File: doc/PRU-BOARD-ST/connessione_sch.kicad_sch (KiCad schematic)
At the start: 1 part, among them J1 Conn_02x25_Top_Bottom

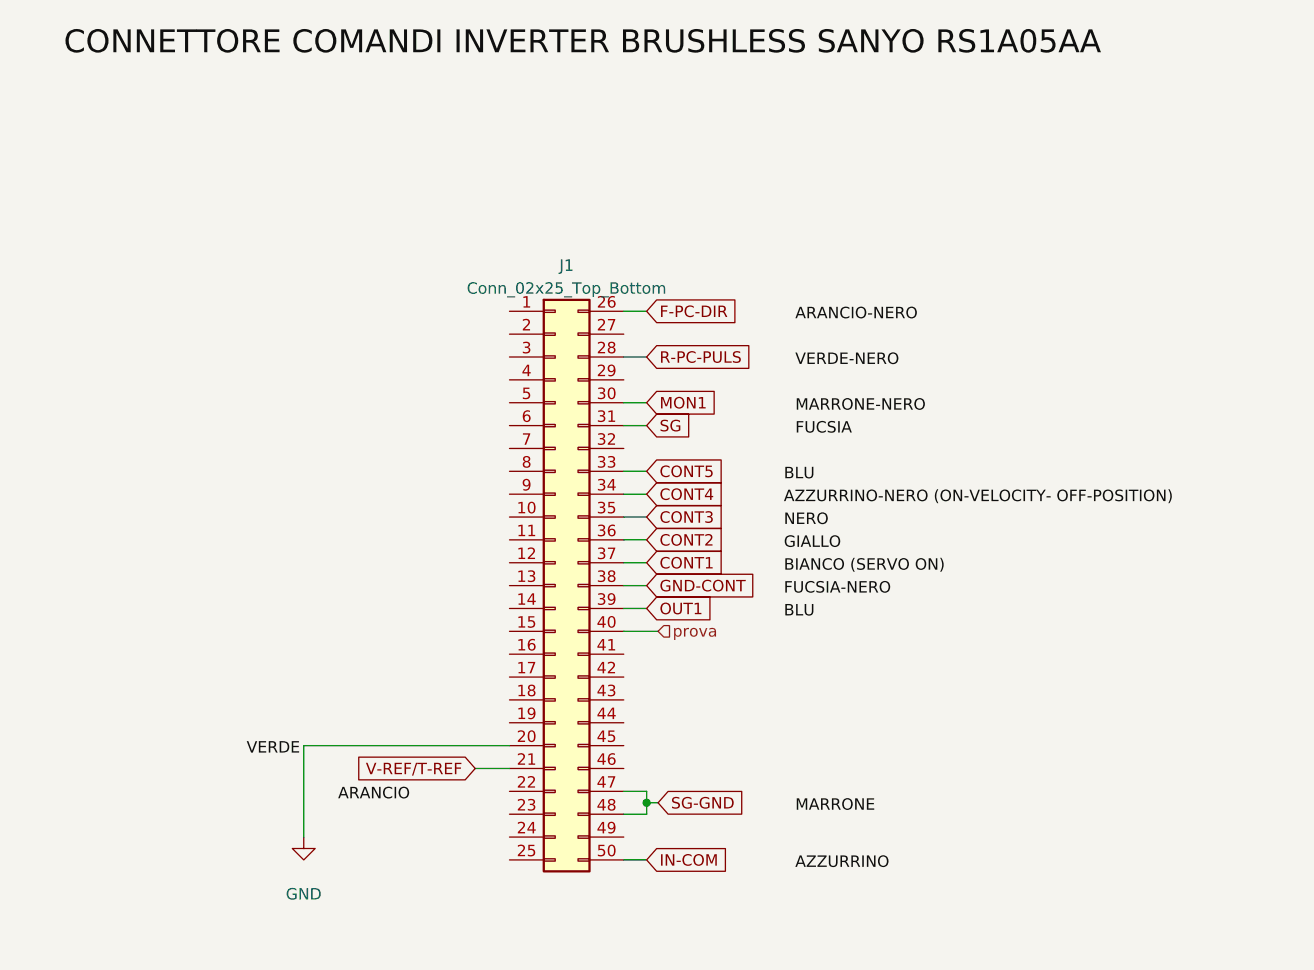
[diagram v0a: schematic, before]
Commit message: 02-2026 - update
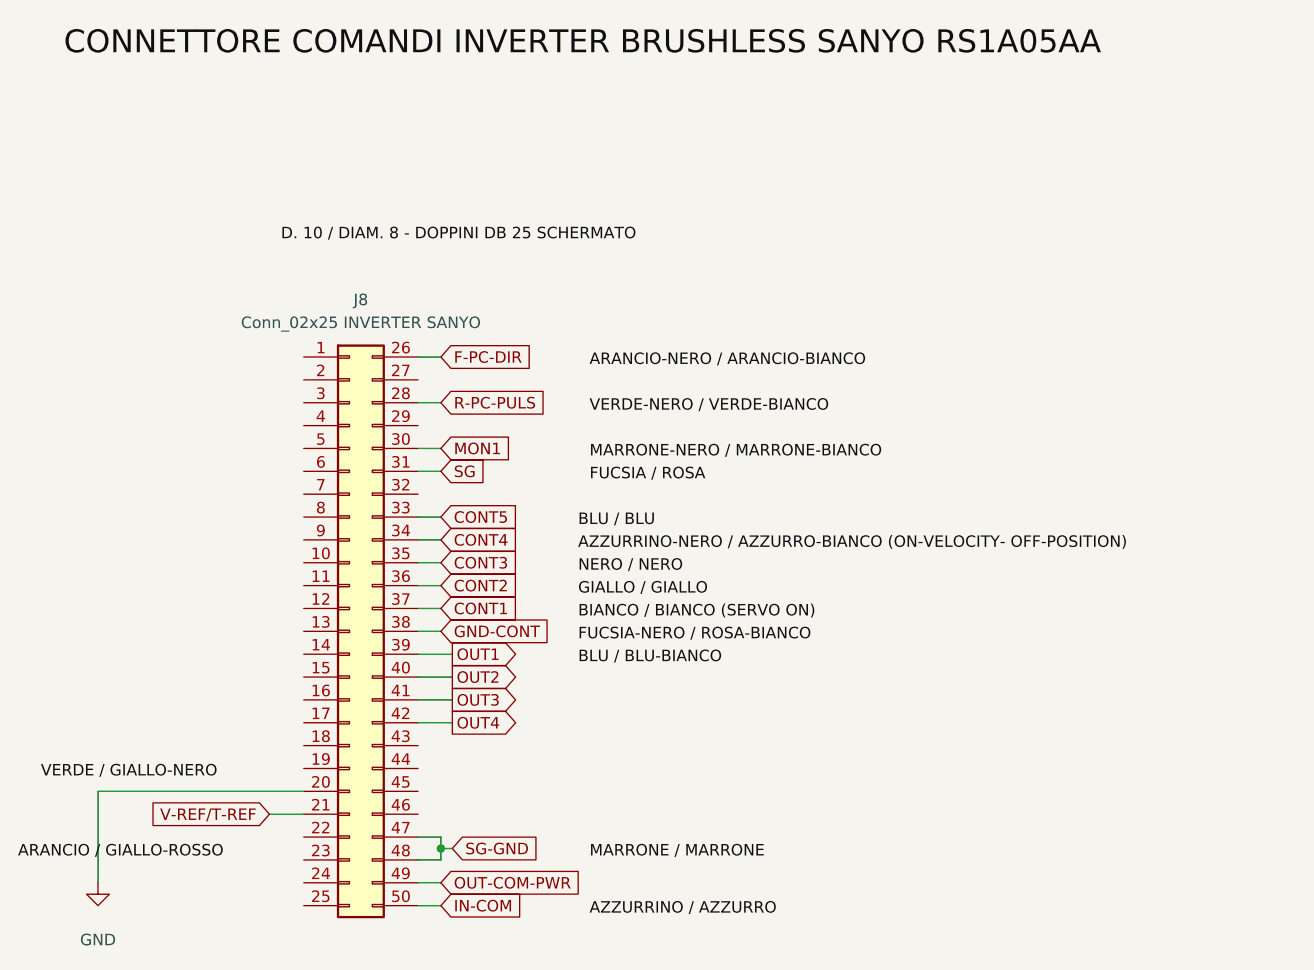
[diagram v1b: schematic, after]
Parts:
- removed J1: Conn_02x25_Top_Bottom, symbol Connector_Generic:Conn_02x25_Top_Bottom
- added J8: Conn_02x25 INVERTER SANYO, symbol Connector_Generic:Conn_02x25_Top_Bottom
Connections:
- net CONT1: now also J8.37 (Pin_37)
- net CONT2: now also J8.36 (Pin_36)
- net CONT3: now also J8.35 (Pin_35)
- net CONT4: now also J8.34 (Pin_34)
- net CONT5: now also J8.33 (Pin_33)
- net F-PC-DIR: now also J8.26 (Pin_26)
- net GND: now also J8.20 (Pin_20)
- net GND-CONT: now also J8.38 (Pin_38)
- net IN-COM: now also J8.50 (Pin_50)
- net MON1: now also J8.30 (Pin_30)
- net OUT1: now also J8.39 (Pin_39)
- net R-PC-PULS: now also J8.28 (Pin_28)
- net SG: now also J8.31 (Pin_31)
- net SG-GND: now also J8.47 (Pin_47), J8.48 (Pin_48)
- net V-REF/T-REF: now also J8.21 (Pin_21)
- new net OUT-COM-PWR: J8.49 (Pin_49)
- new net OUT2: J8.40 (Pin_40)
- new net OUT3: J8.41 (Pin_41)
- new net OUT4: J8.42 (Pin_42)
